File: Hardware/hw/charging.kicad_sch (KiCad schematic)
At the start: 22 parts, among them J1 Screw_Terminal_01x02, Q2 PMOS, Q3 PMOS, Q4 PMOS, Q5 NMOS, Q6 PMOS, U4 SunnyBuddy:PRT-12885, U6 INA219, U7 INA219

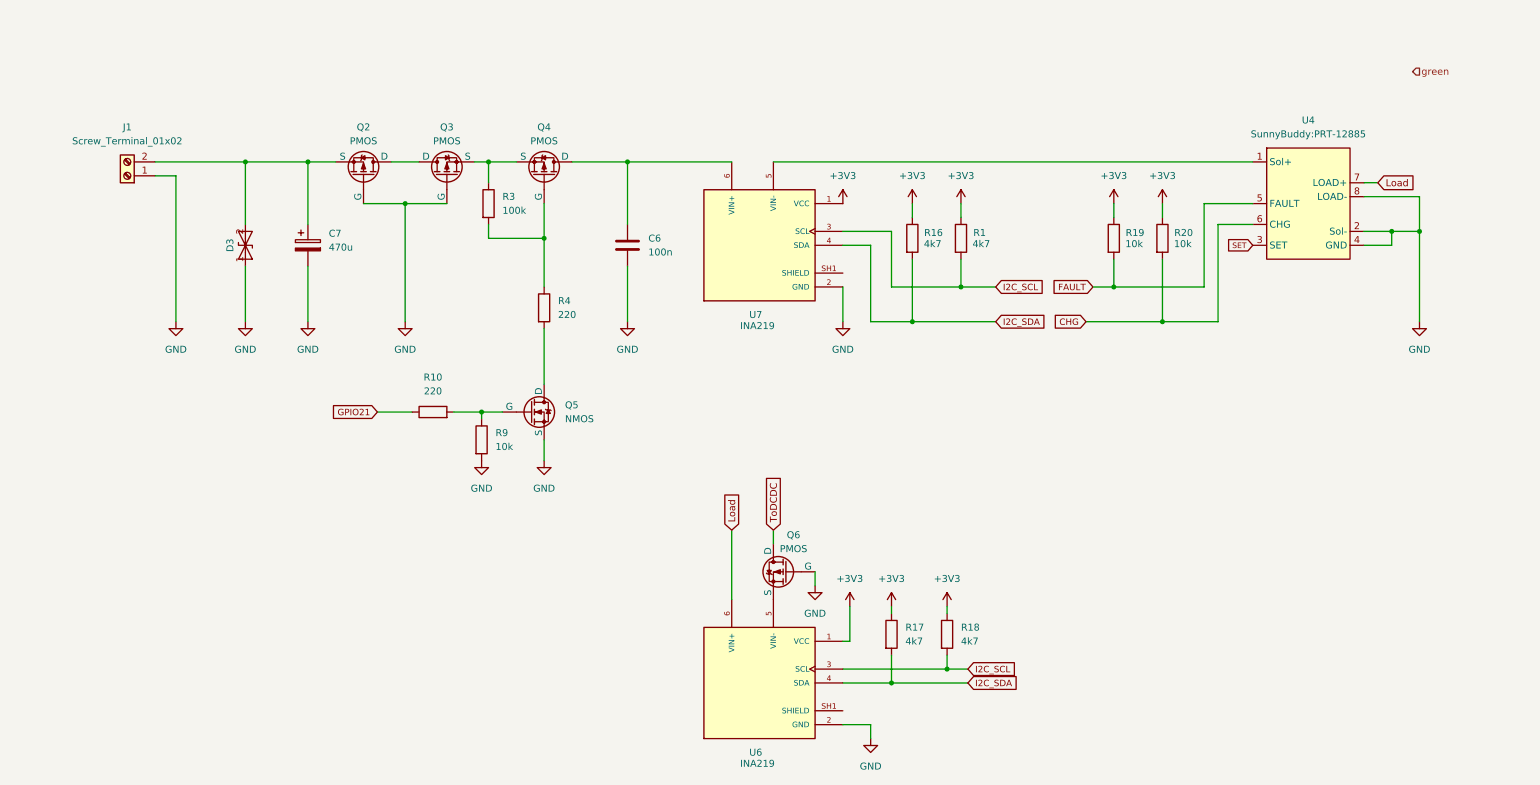
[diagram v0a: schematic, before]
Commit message: Hardware v1.0
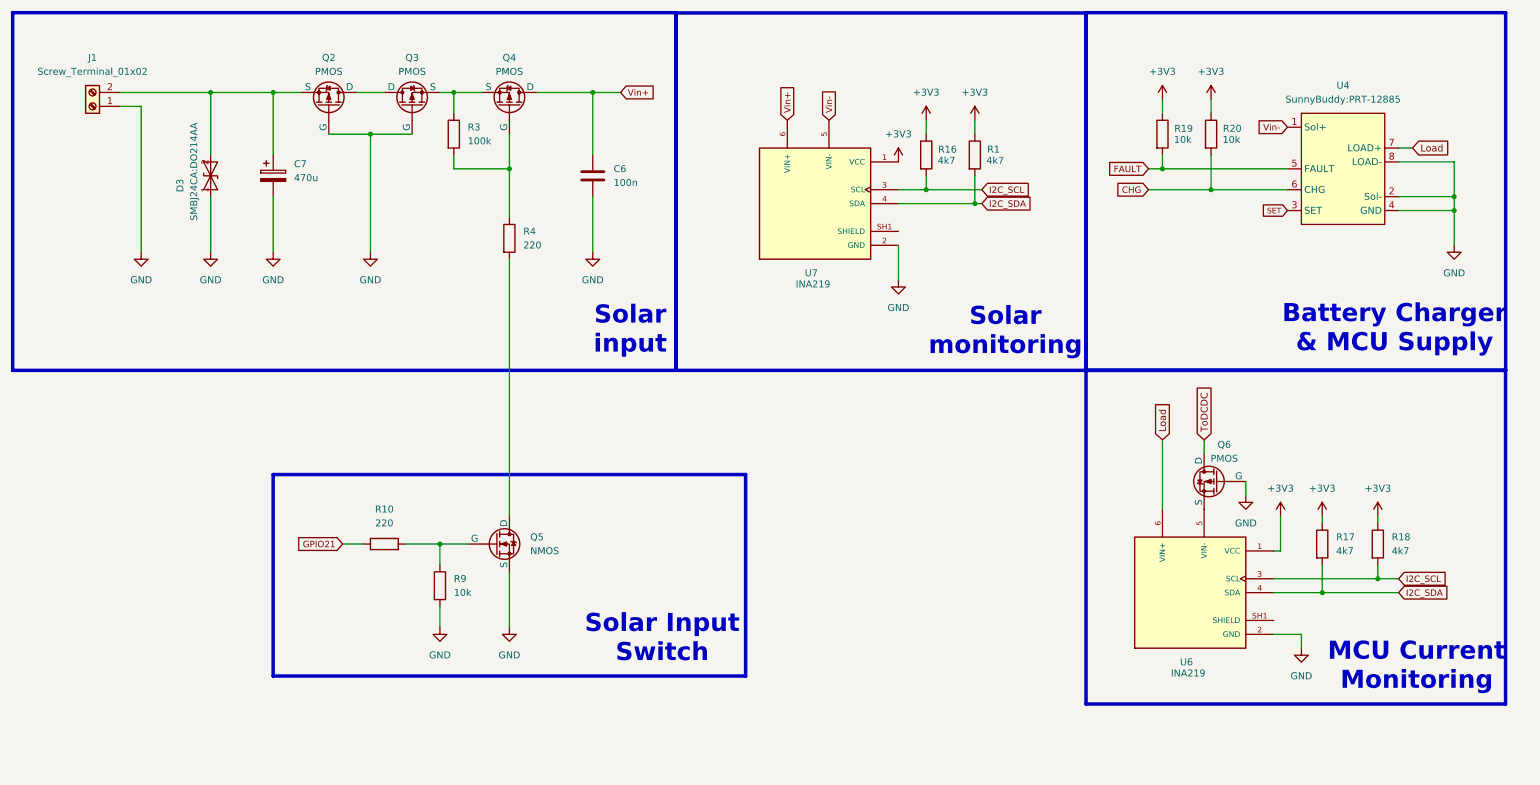
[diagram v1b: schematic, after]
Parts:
- D3: value ~ -> SMBJ24CA:DO214AA
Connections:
- net I2C_SCL: now also R16.2; no longer R1.2
- net I2C_SDA: now also R1.2; no longer R16.2
- net Vin+: now reaches C6.1, Q4.1 (D), U7.6 (VIN+)
- net Vin-: now reaches U4.1 (Sol+), U7.5 (VIN-)
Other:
- note added: "Battery Charger & MCU Supply"
- note added: "MCU Current Monitoring"
- note added: "Solar Input Switch"
- note added: "Solar input"
- note added: "Solar monitoring"
- company: (none) -> UNIZA Faculty of Management Science and Informatics Department of Technical Cybernetics
- title: (none) -> Solar Power Management and Monitoring Circuit
- moved on the sheet: C6, C7, D3, J1, Q2, Q3, Q4, Q5, Q6, R1, R10, R16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

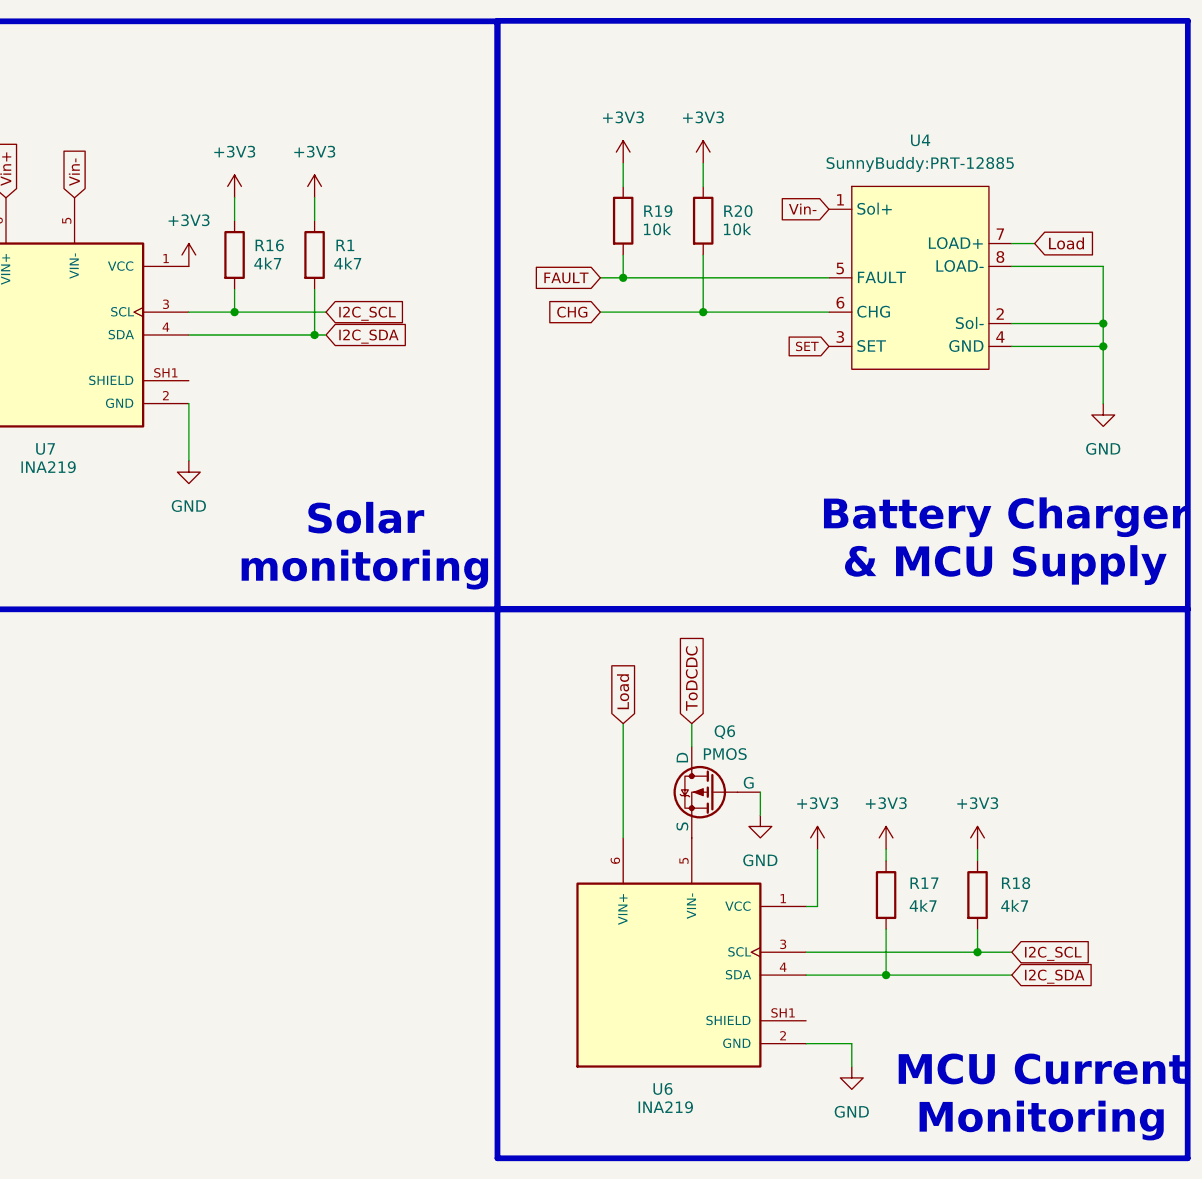
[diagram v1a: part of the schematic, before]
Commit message: External ADC update
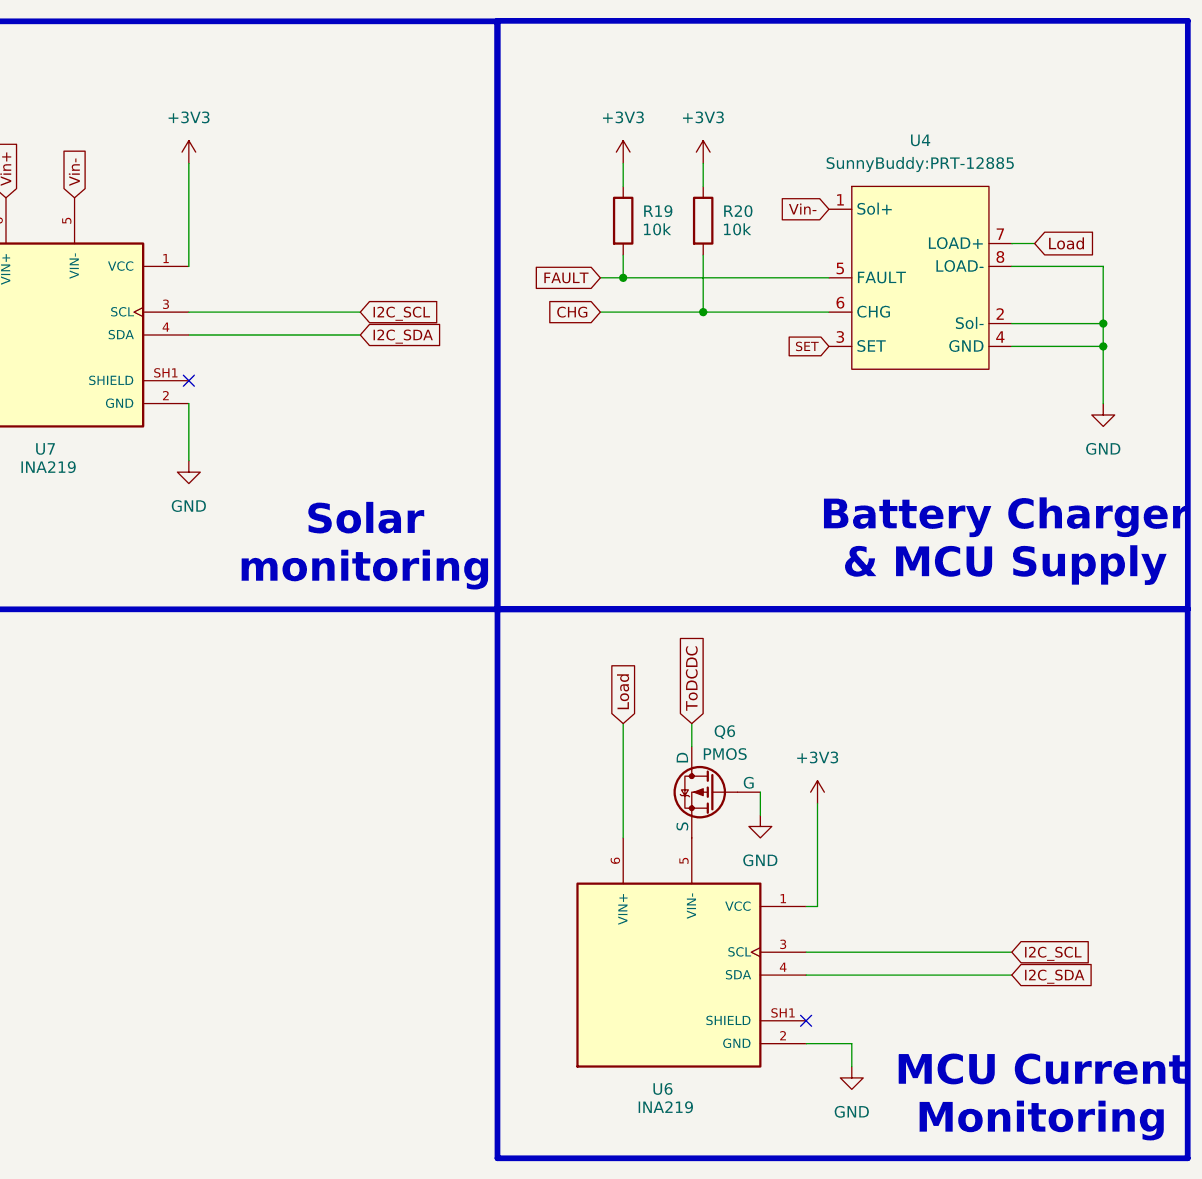
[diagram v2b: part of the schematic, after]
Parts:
- removed R1, R16, R17, R18: 4k7, Resistor_SMD:R_0805_2012Metric, symbol Device:R
- U4: footprint SunnyBuddy:Untitled -> SunnyBuddy:PRT-12885
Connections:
- no-connect marks 0 -> 2

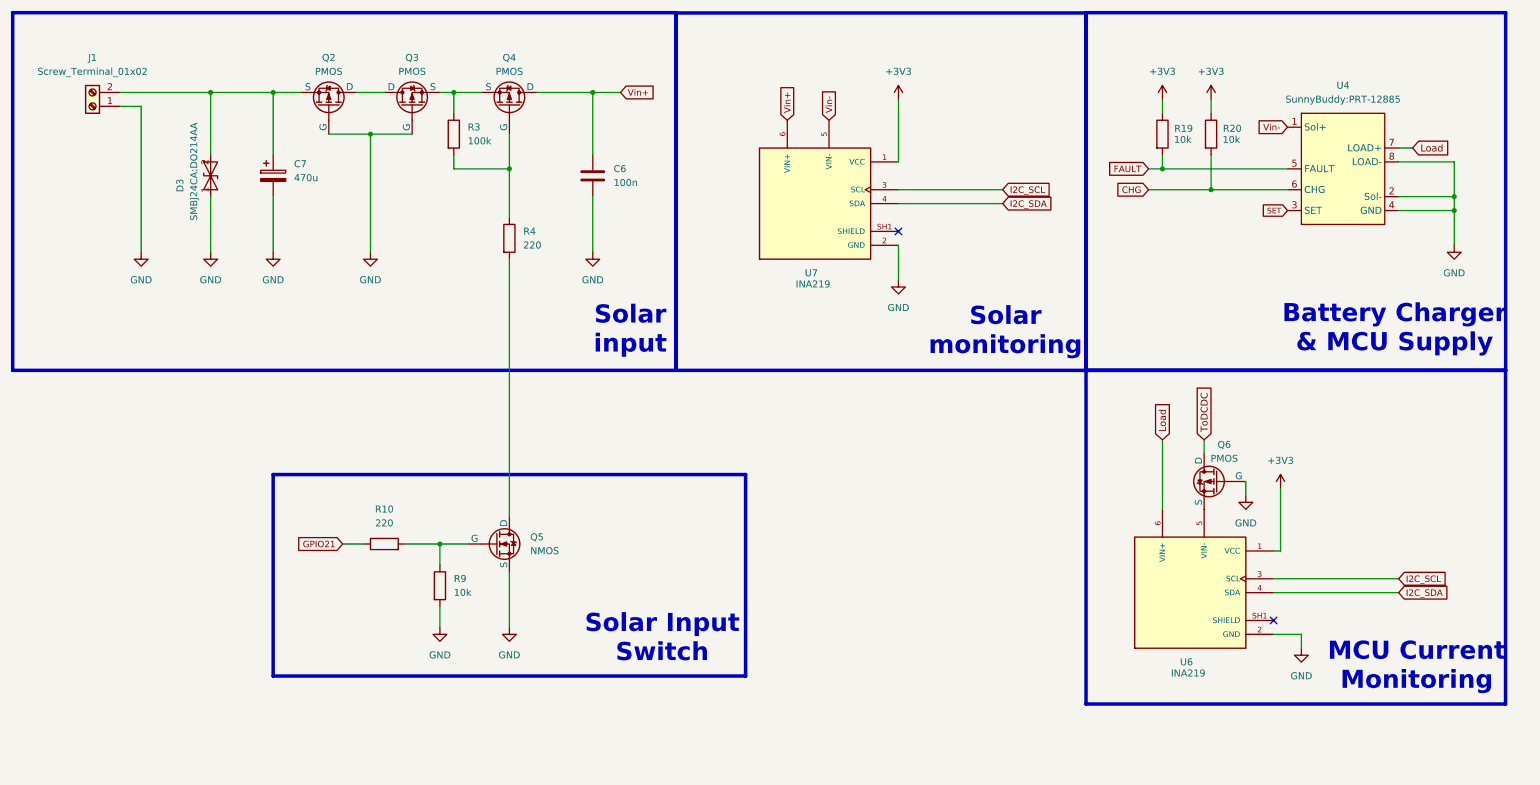
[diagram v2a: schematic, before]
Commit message: Tomáš update
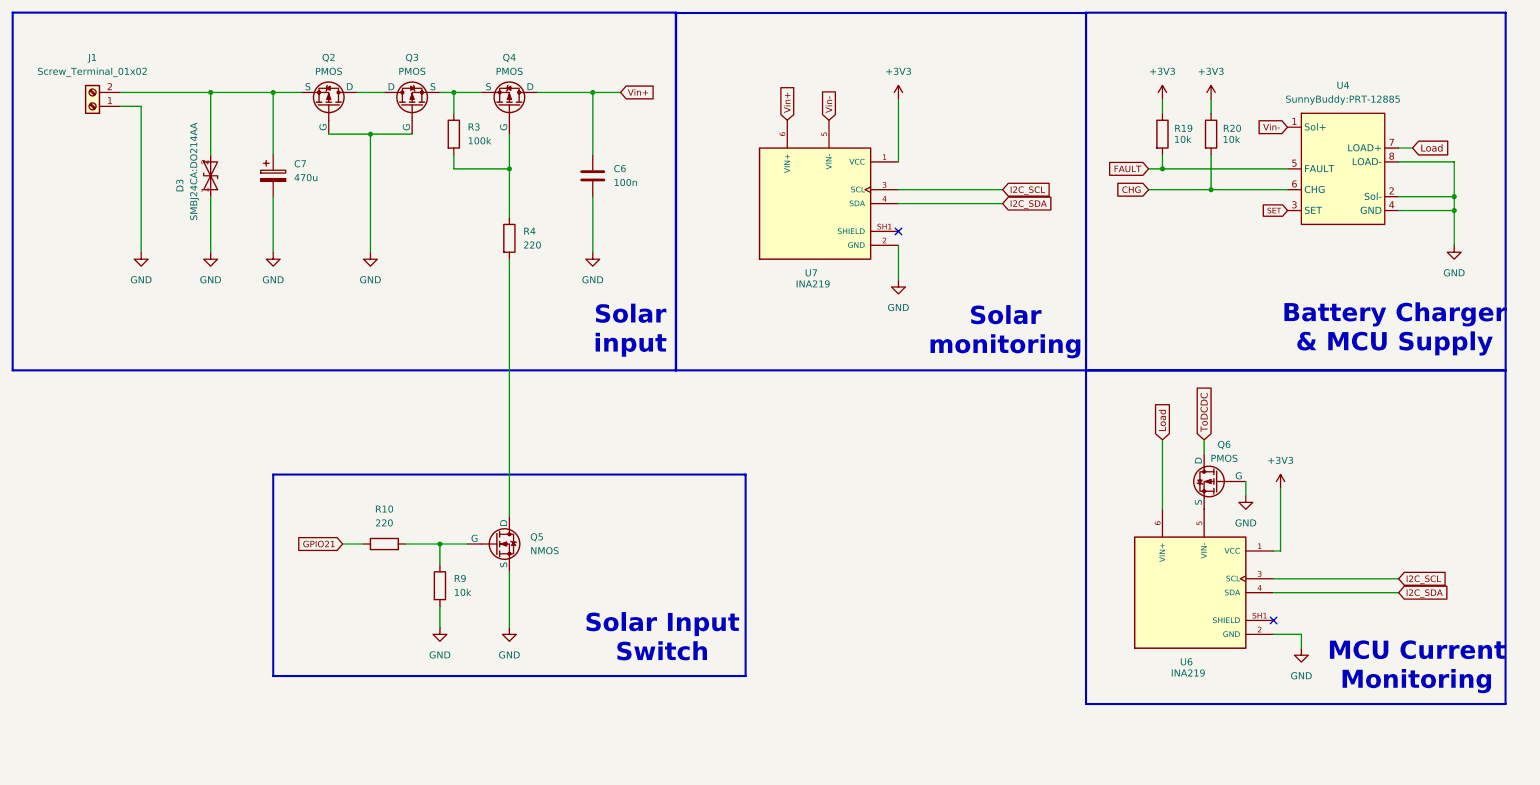
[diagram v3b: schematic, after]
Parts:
- Q5: footprint (none) -> NMOS:SOT95P230X110-3N
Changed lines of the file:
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@@
 		(title "Solar Power Management and Monitoring Circuit")
 		(date "2026-04-24")
-		(rev "Michal Hodoň")
+		(rev "Tomáš Bača")
 		(company "UNIZA Faculty of Management Science and Informatics Department of Technical Cybernetics")
 		(comment 1 "Author: Peter Kolok")
@@
 		(end 146.05 133.35)
 		(stroke
-			(width 0.635)
+			(width 0.381)
 			(type solid)
 		)
@@
 		(end 284.9722 138.467)
 		(stroke
-			(width 0.635)
+			(width 0.381)
 			(type solid)
 		)
@@
 	)
 	(rectangle
-		(start 133.35 12.1377)
+		(start 133.3388 12.1436)
 		(end 208.28 77.47)
 		(stroke
-			(width 0.635)
+			(width 0.381)
 			(type solid)
 		)
@@
 	)
 	(rectangle
-		(start 12.0671 12.0865)
-		(end 133.35 77.47)
-		(stroke
-			(width 0.635)
+		(start 12.0671 12.0754)
+		(end 133.2934 77.47)
+		(stroke
+			(width 0.381)
 			(type solid)
 		)
@@
 		(end 284.9875 77.47)
 		(stroke
-			(width 0.635)
+			(width 0.381)
 			(type solid)
 		)
@@
 			)
 		)
-		(property "Footprint" ""
+		(property "Footprint" "NMOS:SOT95P230X110-3N"
 			(at 105.41 106.68 0)
 			(effects
